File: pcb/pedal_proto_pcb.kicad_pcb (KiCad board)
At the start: 2 copper layers, 100 x 85 mm, 51 parts, among them J1 GND, J10 RV1_2, J11 RV1_1, J12 RV2_3, J13 RV2_2, J14 RV2_1, J15 RV3_3, J16 RV3_2, J17 RV3_1, J18 RV4_3, J19 RV4_2, J2 GND, J20 RV4_1, J21 stomp_A_1, J22 stomp_A_2, J23 stomp_A_3, J24 stomp_B_1, J25 stomp_B_2, J26 stomp_B_3, J27 stomp_C_1, J28 stomp_C_2, J29 stomp_C_3, J3 GND, J30 switch_1, J31 switch_2, J32 switch_3, J33 GND, J34 VDD, J35 LED-, J36 LED+, J37 GND, J38 input, J39 output, J4 GND, J40 GND, J5 Jack-DC, J6 Barrel_Jack_Output, J7 Barrel_Jack_Input, J8 GND, J9 RV1_3, SW1 SW_3PDT, SW2 SW_SPDT, SW3 SW_SPDT

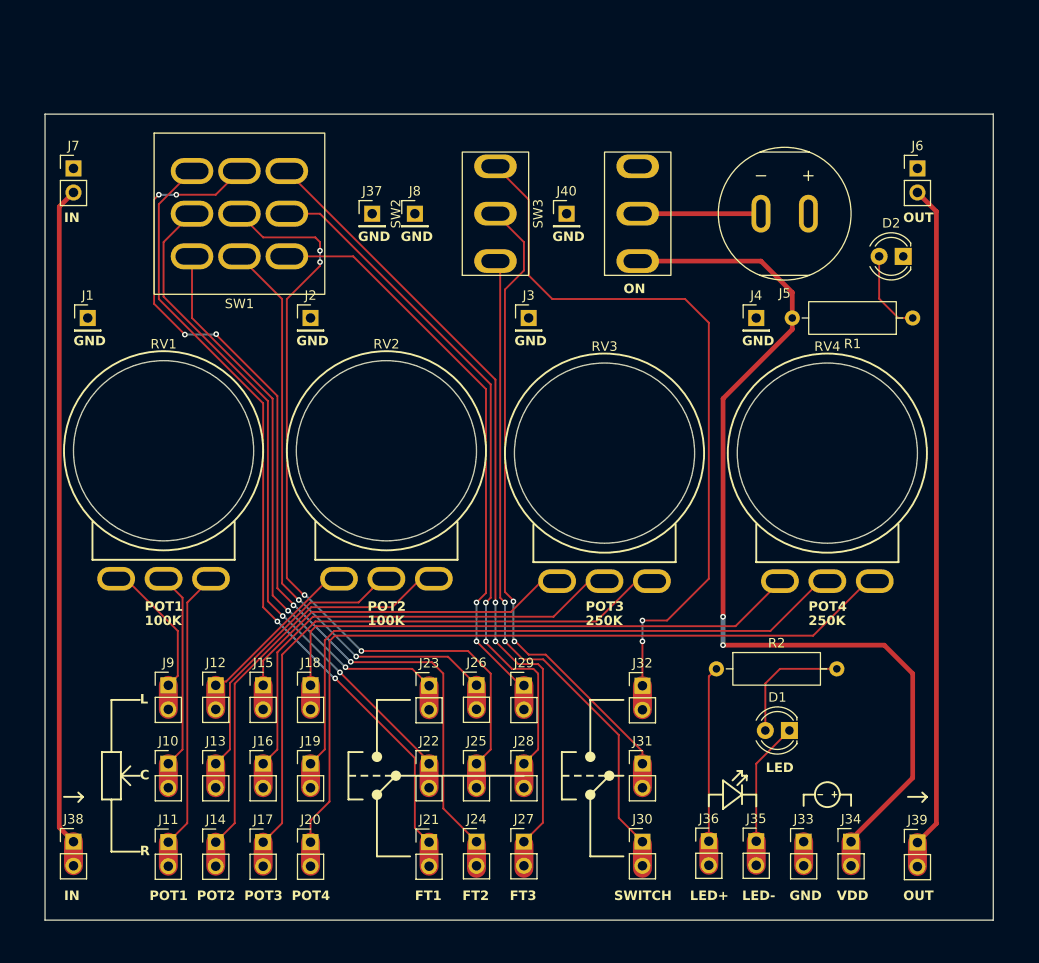
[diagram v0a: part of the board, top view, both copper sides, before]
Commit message: feat: layout done
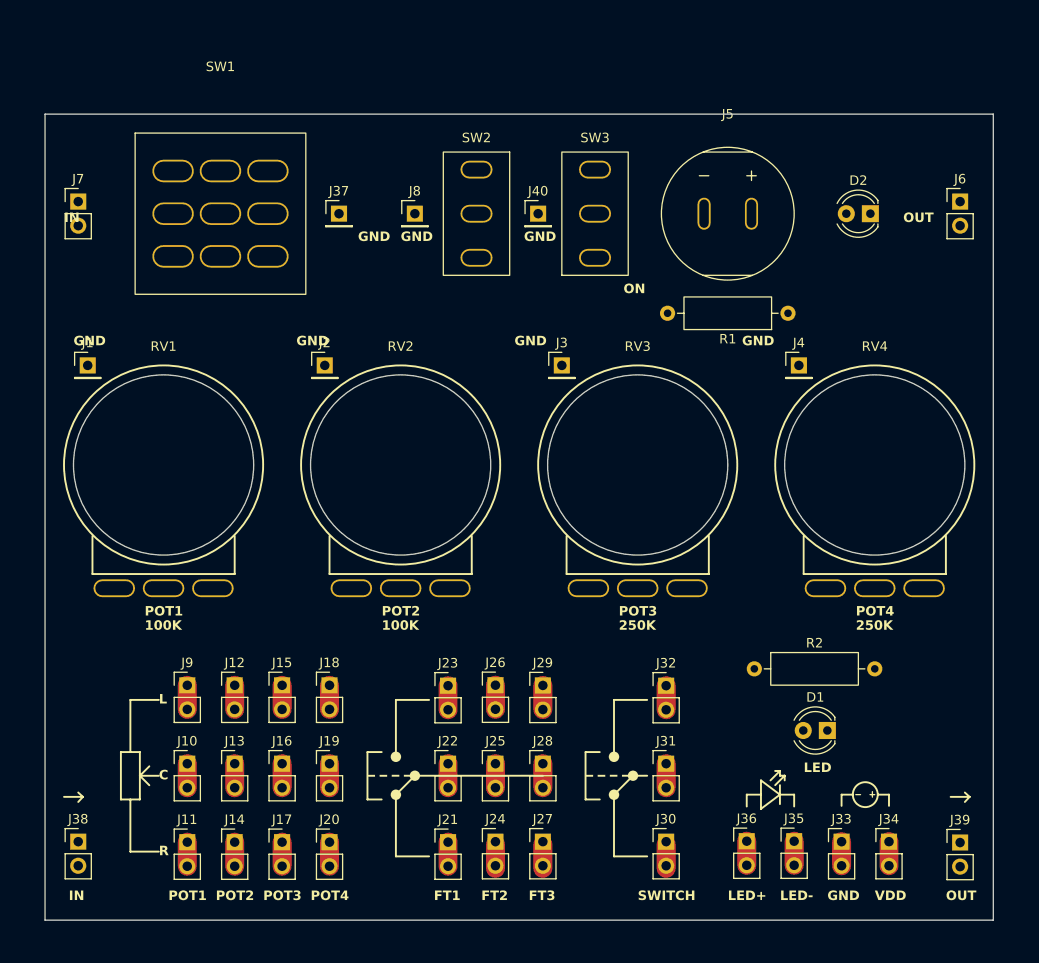
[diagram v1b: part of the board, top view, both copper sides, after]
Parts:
- moved SW2 18.0 mm to (175.0, 82.0), turned to -90 degrees
- moved R1 13.2 mm to (197.8, 92.5)
- moved J4 6.73 mm to (199.0, 98.0)
- moved J3 6.10 mm to (174.0, 98.0)
- moved J5 6.00 mm to (191.5, 72.0)
- moved J6 5.70 mm to (216.0, 80.7)
- moved D2 5.68 mm to (206.5, 82.0)
- moved J2 5.22 mm to (149.0, 98.0)
- moved RV4 5.15 mm to (207.0, 93.5)
- moved J1 5.00 mm to (124.0, 98.0)
- moved J39 4.50 mm to (216.0, 148.3)
- moved SW3 4.50 mm to (167.5, 82.0)
- moved D1 4.00 mm to (202.0, 136.5)
- moved J33 4.00 mm to (203.5, 148.2)
- moved J34 4.00 mm to (208.5, 148.2)
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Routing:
- net Net-(J34-Pin_1): track 102.1 -> 2.54 mm, vias 2 -> 0
- net Net-(J24-Pin_1): track 101.6 -> 2.54 mm, vias 6 -> 0
- net Net-(J21-Pin_1): track 86.6 -> 2.54 mm, vias 2 -> 0
- net Net-(J27-Pin_1): track 86.5 -> 2.54 mm, vias 2 -> 0
- net Net-(J25-Pin_1): track 85.0 -> 2.54 mm, vias 4 -> 0
- net Net-(J20-Pin_1): track 83.1 -> 2.54 mm
- net Net-(J32-Pin_1): track 79.3 -> 2.54 mm, vias 2 -> 0
- net Net-(J28-Pin_1): track 75.9 -> 2.54 mm, vias 2 -> 0
- net Net-(J39-Pin_1): track 72.7 -> 0.00 mm
- net Net-(J38-Pin_1): track 72.2 -> 0.00 mm
- net Net-(J22-Pin_1): track 73.9 -> 3.04 mm, vias 2 -> 0
- net Net-(J30-Pin_1): track 71.4 -> 2.54 mm, vias 2 -> 0
- net Net-(J19-Pin_1): track 71.2 -> 2.54 mm
- net Net-(J31-Pin_1): track 69.7 -> 2.54 mm, vias 2 -> 0
- net Net-(J17-Pin_1): track 63.9 -> 2.54 mm
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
